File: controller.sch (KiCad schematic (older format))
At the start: 18 parts, among them SW1 SW_Push, U2 ATSAMD51J19A, Y1 32.768kHz

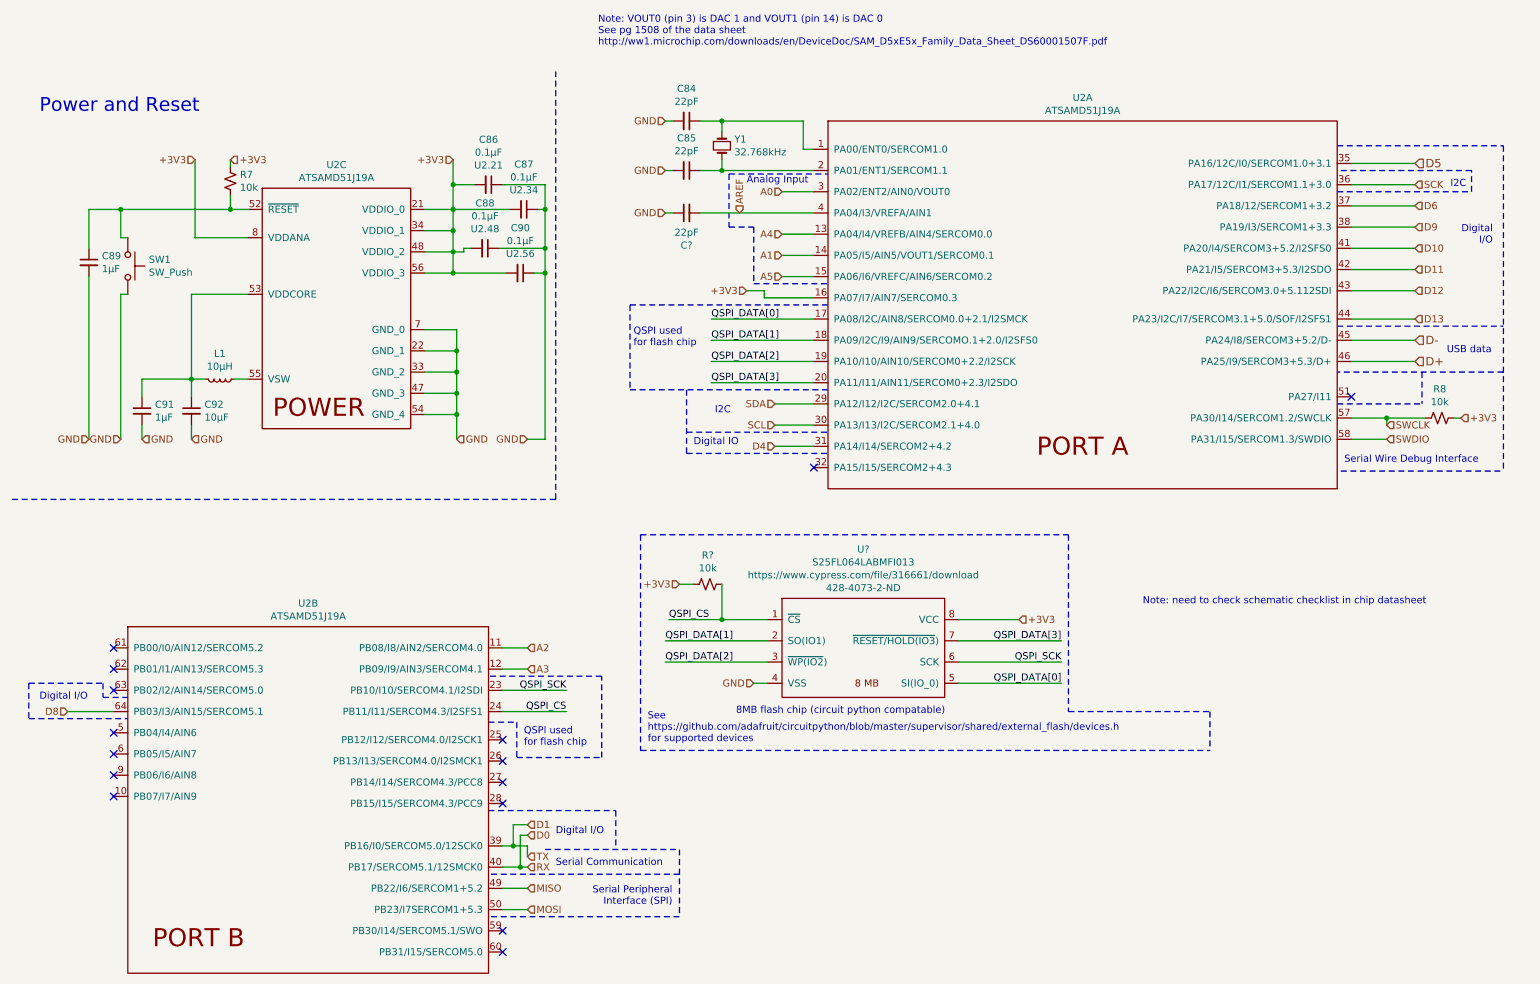
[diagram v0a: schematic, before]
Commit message: update
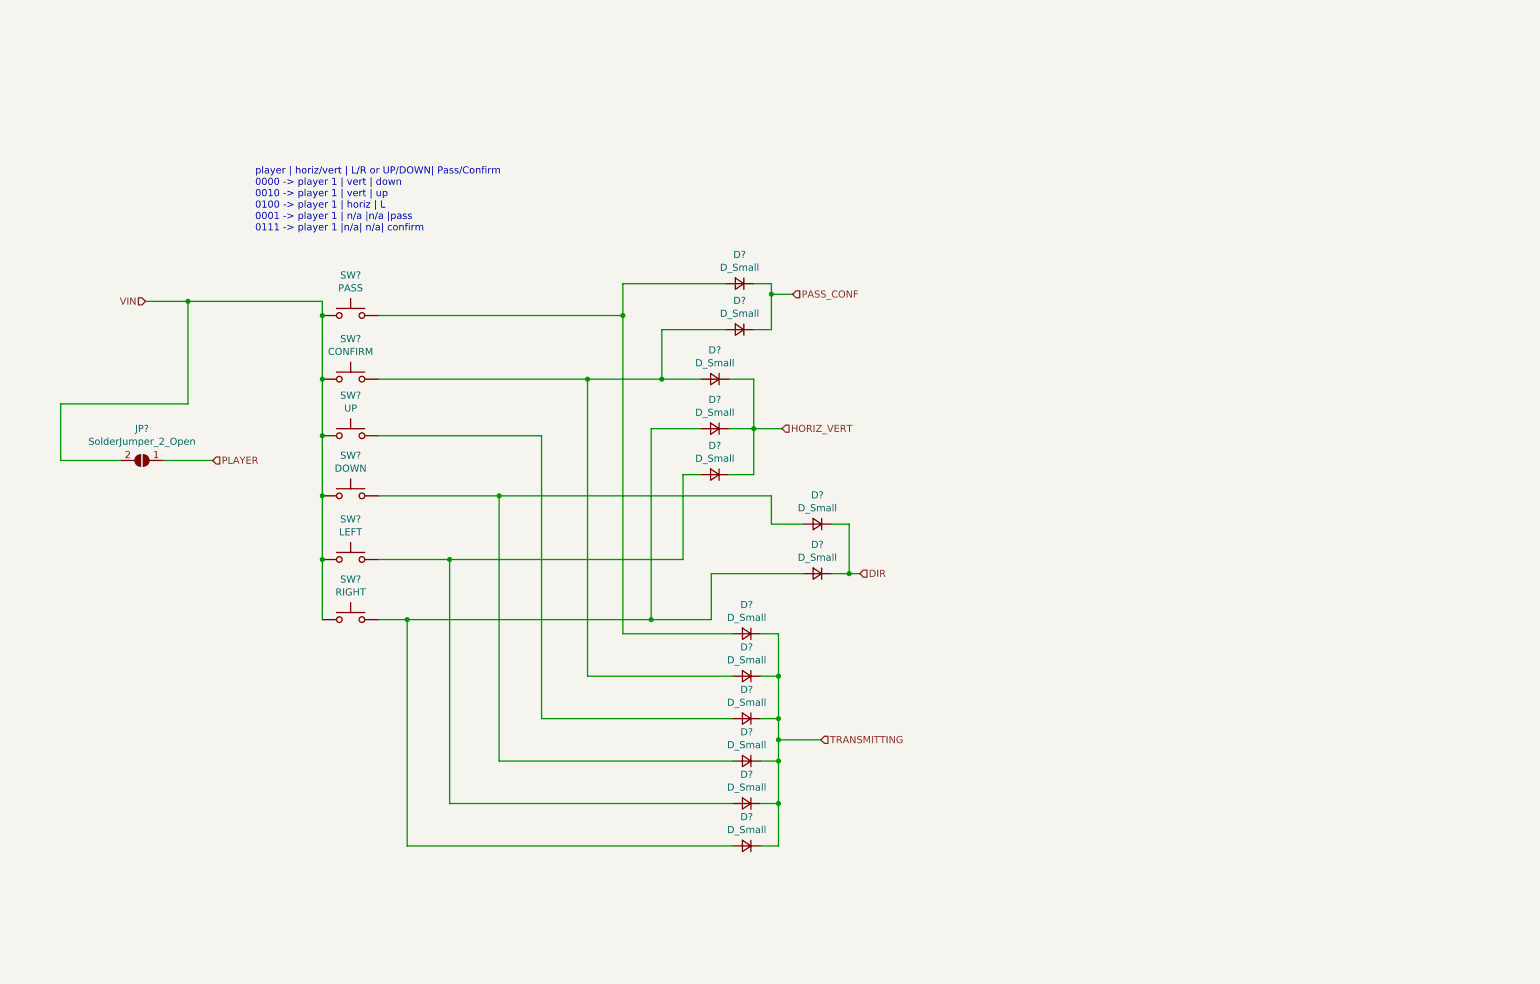
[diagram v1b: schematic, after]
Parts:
- removed C84, C85, C?: 22pF, symbol Device:C_Small
- removed C86, C87, C88, C90: 0.1µF, symbol Device:C_Small
- removed C89, C91: 1µF, symbol Device:C_Small
- removed C92: 10µF, symbol Device:C_Small
- removed L1: 10µH, symbol Device:L_Small
- removed R7, R8, R?: 10k, symbol Device:R_Small_US
- removed SW1: SW_Push, symbol Switch:SW_Push
- removed U2: ATSAMD51J19A, Package_QFP:TQFP-64_10x10mm_P0.5mm, symbol ondine:ATSAMD51J19A
- removed U?: S25FL064LABMFI013, SOIC-8_5.23x5.23mm_P1.27mm, symbol ondine:S25FL064LABMFI013
- removed Y1: 32.768kHz, symbol Device:Crystal_Small
- added D? (x13): D_Small, symbol Device:D_Small
- added JP?: SolderJumper_2_Open, symbol Jumper:SolderJumper_2_Open
- added SW?: CONFIRM, symbol Switch:SW_Push
- added SW?: PASS, symbol Switch:SW_Push
- added SW?: RIGHT, symbol Switch:SW_Push
- added SW?: LEFT, symbol Switch:SW_Push
- added SW?: DOWN, symbol Switch:SW_Push
- added SW?: UP, symbol Switch:SW_Push
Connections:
- new net: D?.2 (A), D?.2 (A), D?.2 (A), SW?.2 (x2)
- new net: D?.2 (A), D?.2 (A), SW?.2 (x3)
- new net: D?.2 (A), SW?.2
- new net DIR: D?.1 (K), D?.1 (K)
- new net HORIZ_VERT: D?.1 (K), D?.1 (K), D?.1 (K)
- new net PASS_CONF: D?.1 (K), D?.1 (K)
- new net PLAYER: JP?.1 (A)
- new net TRANSMITTING: D?.1 (K), D?.1 (K), D?.1 (K), D?.1 (K), D?.1 (K), D?.1 (K)
- new net VIN: JP?.2 (B), SW?.1, SW?.1, SW?.1, SW?.1, SW?.1, SW?.1
- no-connect marks 15 -> 0
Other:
- note added: "player | horiz/vert | L/R or UP/DOWN| Pass/Confirm\n0000 -> player 1 | vert | down\n0010 -> player 1 | vert | up\n0100 -> player 1 | horiz | L\n0001 -> player 1 | n/a |n/a |pass\n0111 -> player 1 |n/a| n/a| confirm\n\n\n"
- note removed: "8MB flash chip (circuit python compatable)\n"
- note removed: "Analog Input\n"
- note removed: "Digital I/O"
- note removed: "Digital I/O\n"
- note removed: "Digital IO"
- note removed: "Digital\nI/O"
- note removed: "I2C"
- note removed: "Note: VOUT0 (pin 3) is DAC 1 and VOUT1 (pin 14) is DAC 0\nSee pg 1508 of the data sheet\nhttp://ww1.microchip.com/downloads/en/DeviceDoc/SAM_D5xE5x_Family_Data_Sheet_DS60001507F.pdf"
- note removed: "Note: need to check schematic checklist in chip datasheet"
- note removed: "Power and Reset"
- note removed: "QSPI used \nfor flash chip\n"
- note removed: "See \nhttps://github.com/adafruit/circuitpython/blob/master/supervisor/shared/external_flash/devices.h \nfor supported devices"
- note removed: "Serial Communication"
- note removed: "Serial Peripheral\nInterface (SPI)"
- note removed: "Serial Wire Debug Interface"
- note removed: "USB data"
